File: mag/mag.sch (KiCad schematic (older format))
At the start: 24 parts, among them K1 кнопка_FSMSM, K2 кнопка_FSMSM

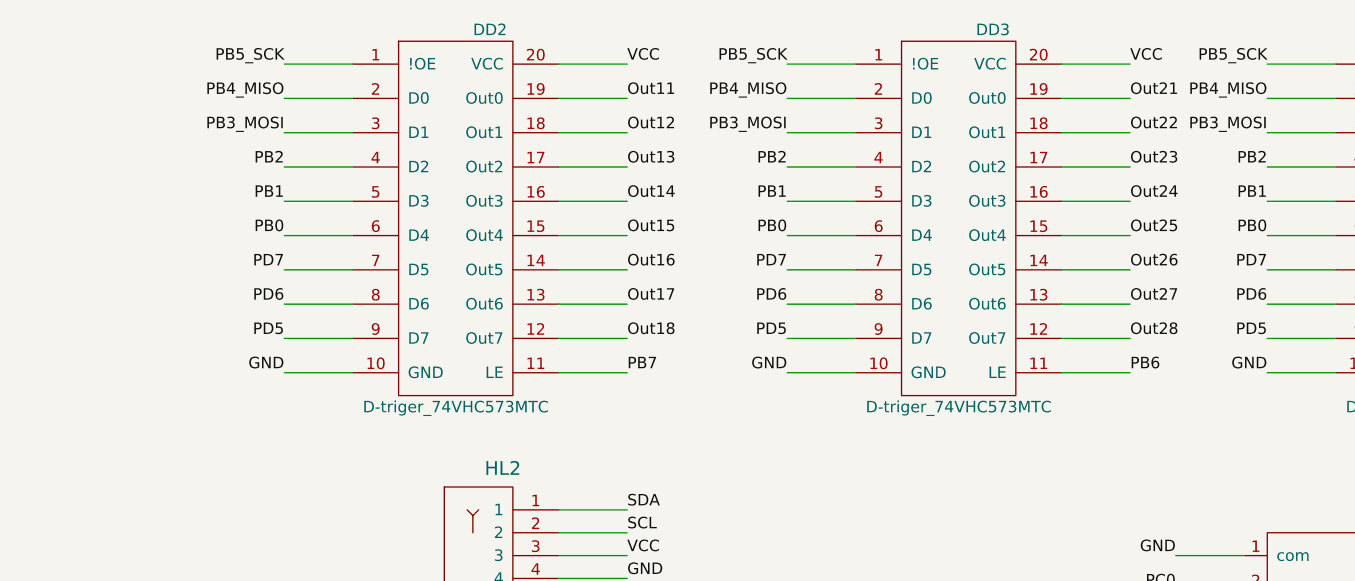
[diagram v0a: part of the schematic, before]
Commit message: закончена трассировка и маркировка
не подготавливались файлы производства
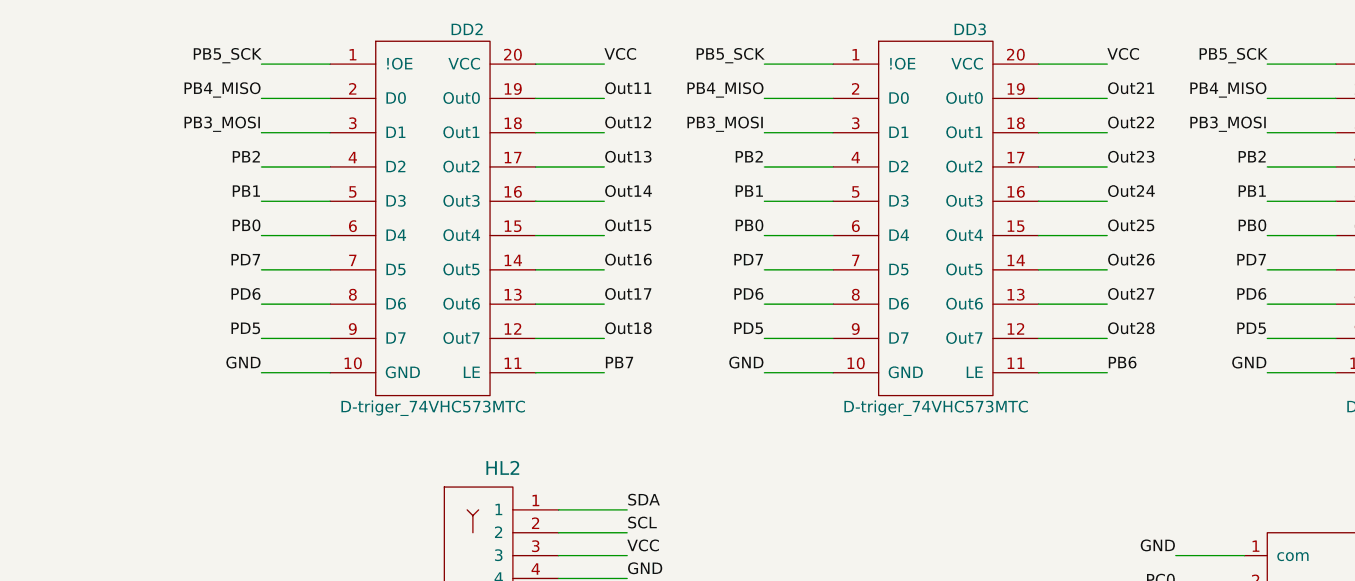
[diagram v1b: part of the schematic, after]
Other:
- moved on the sheet: DD2, DD3
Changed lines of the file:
@@
 L elements:D-triger_8bit DD2
 U 1 1 5CE49B21
-P 8200 950
-F 0 "DD2" H 8600 1100 50  0000 C CNN
-F 1 "D-triger_74VHC573MTC" H 8450 -550 50  0000 C CNN
-F 2 "N_DD:SSOP-20" H 8200 950 50  0001 C CNN
-F 3 "" H 8200 950 50  0001 C CNN
-	1    8200 950
+P 8100 950
+F 0 "DD2" H 8500 1100 50  0000 C CNN
+F 1 "D-triger_74VHC573MTC" H 8350 -550 50  0000 C CNN
+F 2 "N_DD:SSOP-20" H 8100 950 50  0001 C CNN
+F 3 "" H 8100 950 50  0001 C CNN
+	1    8100 950
 	1    0    0    -1
 $EndComp
@@
 PB2
 Wire Wire Line
-	8000 1100 7700 1100
-Wire Wire Line
-	8000 1250 7700 1250
-Wire Wire Line
-	8000 1400 7700 1400
-Wire Wire Line
-	8000 1550 7700 1550
-Wire Wire Line
-	8000 1700 7700 1700
-Wire Wire Line
-	8000 1850 7700 1850
-Wire Wire Line
-	8000 2000 7700 2000
-Wire Wire Line
-	8000 2150 7700 2150
+	7900 1100 7600 1100
+Wire Wire Line
+	7900 1250 7600 1250
+Wire Wire Line
+	7900 1400 7600 1400
+Wire Wire Line
+	7900 1550 7600 1550
+Wire Wire Line
+	7900 1700 7600 1700
+Wire Wire Line
+	7900 1850 7600 1850
+Wire Wire Line
+	7900 2000 7600 2000
+Wire Wire Line
+	7900 2150 7600 2150
 Wire Wire Line
 	3200 3600 2900 3600
@@
 VCC
 Wire Wire Line
-	8000 2300 7700 2300
-Text Label 7700 2300 2    50   ~ 0
-GND
-Wire Wire Line
-	9200 950  8900 950
-Text Label 9200 950  0    50   ~ 0
-VCC
-Wire Wire Line
-	8000 950  7700 950
+	7900 2300 7600 2300
+Text Label 7600 2300 2    50   ~ 0
+GND
+Wire Wire Line
+	9100 950  8800 950
+Text Label 9100 950  0    50   ~ 0
+VCC
+Wire Wire Line
+	7900 950  7600 950
 Wire Wire Line
 	8900 2900 9200 2900
@@
 L elements:D-triger_8bit DD3
 U 1 1 5CE59956
-P 10400 950
-F 0 "DD3" H 10800 1100 50  0000 C CNN
-F 1 "D-triger_74VHC573MTC" H 10650 -550 50  0000 C CNN
-F 2 "N_DD:SSOP-20" H 10400 950 50  0001 C CNN
-F 3 "" H 10400 950 50  0001 C CNN
-	1    10400 950
-	1    0    0    -1
-$EndComp
-Wire Wire Line
-	10200 1100 9900 1100
-Wire Wire Line
-	10200 1250 9900 1250
-Wire Wire Line
-	10200 1400 9900 1400
-Wire Wire Line
-	10200 1550 9900 1550
-Wire Wire Line
-	10200 1700 9900 1700
-Wire Wire Line
-	10200 1850 9900 1850
-Wire Wire Line
-	10200 2000 9900 2000
-Wire Wire Line
-	10200 2150 9900 2150
-Wire Wire Line
-	10200 2300 9900 2300
-Wire Wire Line
-	11400 950  11100 950
-Text Label 11400 950  0    50   ~ 0
-VCC
-Wire Wire Line
-	10200 950  9900 950
+P 10300 950
+F 0 "DD3" H 10700 1100 50  0000 C CNN
+F 1 "D-triger_74VHC573MTC" H 10550 -550 50  0000 C CNN
+F 2 "N_DD:SSOP-20" H 10300 950 50  0001 C CNN
+F 3 "" H 10300 950 50  0001 C CNN
+	1    10300 950
+	1    0    0    -1
+$EndComp
+Wire Wire Line
+	10100 1100 9800 1100
+Wire Wire Line
+	10100 1250 9800 1250
+Wire Wire Line
+	10100 1400 9800 1400
+Wire Wire Line
+	10100 1550 9800 1550
+Wire Wire Line
+	10100 1700 9800 1700
+Wire Wire Line
+	10100 1850 9800 1850
+Wire Wire Line
+	10100 2000 9800 2000
+Wire Wire Line
+	10100 2150 9800 2150
+Wire Wire Line
+	10100 2300 9800 2300
+Wire Wire Line
+	11300 950  11000 950
+Text Label 11300 950  0    50   ~ 0
+VCC
+Wire Wire Line
+	10100 950  9800 950
 $Comp
 L elements:D-triger_8bit DD4
@@
 NoConn ~ 13450 4900
 Wire Wire Line
-	9200 1100 8900 1100
-Text Label 9200 1100 0    50   ~ 0
+	9100 1100 8800 1100
+Text Label 9100 1100 0    50   ~ 0
 Out11
 Wire Wire Line
-	9200 1250 8900 1250
-Text Label 9200 1250 0    50   ~ 0
+	9100 1250 8800 1250
+Text Label 9100 1250 0    50   ~ 0
 Out12
 Wire Wire Line
-	9200 1400 8900 1400
-Text Label 9200 1400 0    50   ~ 0
+	9100 1400 8800 1400
+Text Label 9100 1400 0    50   ~ 0
 Out13
 Wire Wire Line
-	9200 1550 8900 1550
-Text Label 9200 1550 0    50   ~ 0
+	9100 1550 8800 1550
+Text Label 9100 1550 0    50   ~ 0
 Out14
 Wire Wire Line
-	9200 1700 8900 1700
-Text Label 9200 1700 0    50   ~ 0
+	9100 1700 8800 1700
+Text Label 9100 1700 0    50   ~ 0
 Out15
 Wire Wire Line
-	9200 1850 8900 1850
-Text Label 9200 1850 0    50   ~ 0
+	9100 1850 8800 1850
+Text Label 9100 1850 0    50   ~ 0
 Out16
 Wire Wire Line
-	9200 2000 8900 2000
-Text Label 9200 2000 0    50   ~ 0
+	9100 2000 8800 2000
+Text Label 9100 2000 0    50   ~ 0
 Out17
 Wire Wire Line
-	9200 2150 8900 2150
-Text Label 9200 2150 0    50   ~ 0
+	9100 2150 8800 2150
+Text Label 9100 2150 0    50   ~ 0
 Out18
 Wire Wire Line
-	11400 1100 11100 1100
-Text Label 11400 1100 0    50   ~ 0
+	11300 1100 11000 1100
+Text Label 11300 1100 0    50   ~ 0
 Out21
 Wire Wire Line
-	11400 1250 11100 1250
-Text Label 11400 1250 0    50   ~ 0
+	11300 1250 11000 1250
+Text Label 11300 1250 0    50   ~ 0
 Out22
 Wire Wire Line
-	11400 1400 11100 1400
-Text Label 11400 1400 0    50   ~ 0
+	11300 1400 11000 1400
+Text Label 11300 1400 0    50   ~ 0
 Out23
 Wire Wire Line
-	11400 1550 11100 1550
-Text Label 11400 1550 0    50   ~ 0
+	11300 1550 11000 1550
+Text Label 11300 1550 0    50   ~ 0
 Out24
 Wire Wire Line
-	11400 1700 11100 1700
-Text Label 11400 1700 0    50   ~ 0
+	11300 1700 11000 1700
+Text Label 11300 1700 0    50   ~ 0
 Out25
 Wire Wire Line
-	11400 1850 11100 1850
-Text Label 11400 1850 0    50   ~ 0
+	11300 1850 11000 1850
+Text Label 11300 1850 0    50   ~ 0
 Out26
 Wire Wire Line
-	11400 2000 11100 2000
-Text Label 11400 2000 0    50   ~ 0
+	11300 2000 11000 2000
+Text Label 11300 2000 0    50   ~ 0
 Out27
 Wire Wire Line
-	11400 2150 11100 2150
-Text Label 11400 2150 0    50   ~ 0
+	11300 2150 11000 2150
+Text Label 11300 2150 0    50   ~ 0
 Out28
 Wire Wire Line
@@
 	13500 2300 13200 2300
 Wire Wire Line
-	11400 2300 11100 2300
-Wire Wire Line
-	9200 2300 8900 2300
+	11300 2300 11000 2300
+Wire Wire Line
+	9100 2300 8800 2300
 $Comp
 L elements:кнопка K1
@@
 Text Label 13750 4450 0    50   ~ 0
 Out27
-Text Label 7700 1250 2    50   ~ 0
+Text Label 7600 1250 2    50   ~ 0
 PB3_MOSI
-Text Label 7700 2150 2    50   ~ 0
+Text Label 7600 2150 2    50   ~ 0
 PD5
-Text Label 7700 2000 2    50   ~ 0
+Text Label 7600 2000 2    50   ~ 0
 PD6
-Text Label 7700 1850 2    50   ~ 0
+Text Label 7600 1850 2    50   ~ 0
 PD7
-Text Label 7700 1700 2    50   ~ 0
+Text Label 7600 1700 2    50   ~ 0
 PB0
-Text Label 7700 1550 2    50   ~ 0
+Text Label 7600 1550 2    50   ~ 0
 PB1
-Text Label 7700 1400 2    50   ~ 0
+Text Label 7600 1400 2    50   ~ 0
 PB2
-Text Label 7700 1100 2    50   ~ 0
+Text Label 7600 1100 2    50   ~ 0
 PB4_MISO
-Text Label 7700 950  2    50   ~ 0
+Text Label 7600 950  2    50   ~ 0
 PB5_SCK
-Text Label 9900 2300 2    50   ~ 0
-GND
-Text Label 9900 1250 2    50   ~ 0
+Text Label 9800 2300 2    50   ~ 0
+GND
+Text Label 9800 1250 2    50   ~ 0
 PB3_MOSI
-Text Label 9900 2150 2    50   ~ 0
+Text Label 9800 2150 2    50   ~ 0
 PD5
-Text Label 9900 2000 2    50   ~ 0
+Text Label 9800 2000 2    50   ~ 0
 PD6
-Text Label 9900 1850 2    50   ~ 0
+Text Label 9800 1850 2    50   ~ 0
 PD7
-Text Label 9900 1700 2    50   ~ 0
+Text Label 9800 1700 2    50   ~ 0
 PB0
-Text Label 9900 1550 2    50   ~ 0
+Text Label 9800 1550 2    50   ~ 0
 PB1
-Text Label 9900 1400 2    50   ~ 0
+Text Label 9800 1400 2    50   ~ 0
 PB2
-Text Label 9900 1100 2    50   ~ 0
+Text Label 9800 1100 2    50   ~ 0
 PB4_MISO
-Text Label 9900 950  2    50   ~ 0
+Text Label 9800 950  2    50   ~ 0
 PB5_SCK
 Text Label 12000 2300 2    50   ~ 0
@@
 Text Label 2900 4000 2    50   ~ 0
 PB6
-Text Label 11400 2300 0    50   ~ 0
+Text Label 11300 2300 0    50   ~ 0
 PB6
-Text Label 9200 2300 0    50   ~ 0
+Text Label 9100 2300 0    50   ~ 0
 PB7
 Text Label 2900 4100 2    50   ~ 0
